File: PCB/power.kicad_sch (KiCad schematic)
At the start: 9 parts, among them SW1 SW_SPDT, U4 RT9013-33GB

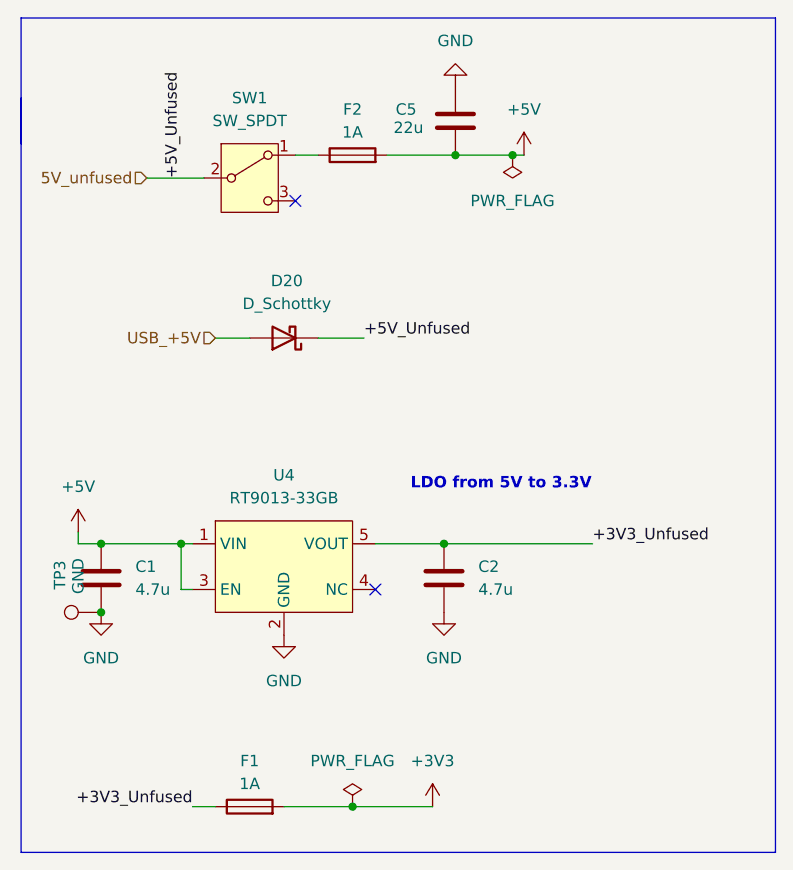
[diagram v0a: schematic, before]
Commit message: init layout
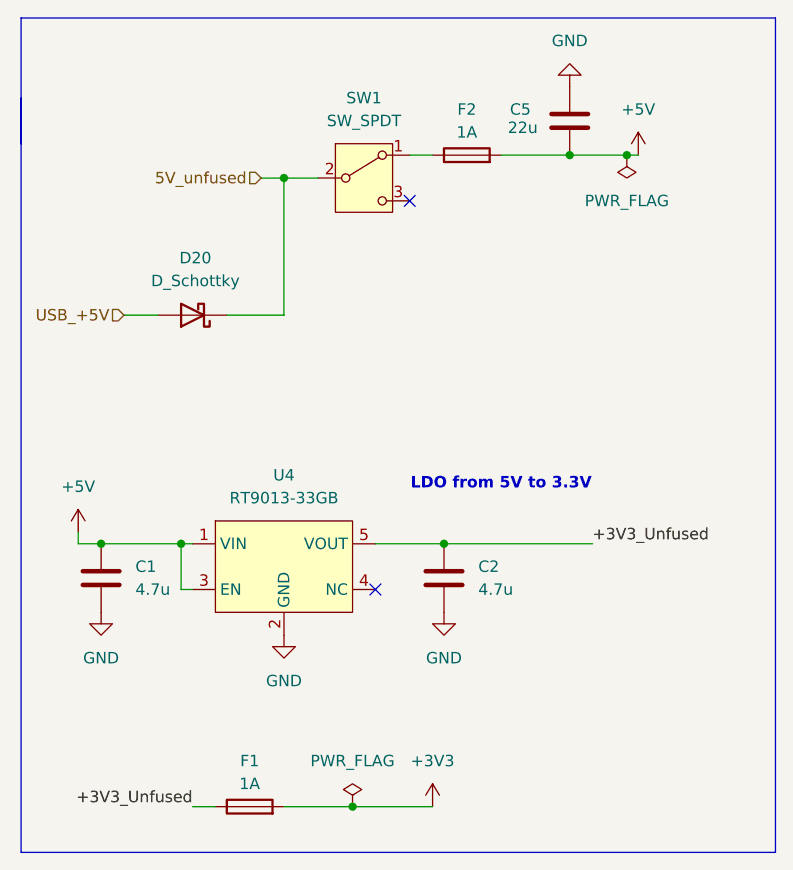
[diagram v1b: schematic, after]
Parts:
- removed TP3: GND, TestPoint:TestPoint_THTPad_1.5x1.5mm_Drill0.7mm, symbol Connector:TestPoint
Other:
- moved on the sheet: C5, D20, F2, SW1
